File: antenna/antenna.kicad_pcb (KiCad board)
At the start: 2 copper layers, 50 x 43.3 mm, 24 parts, among them J1 Conn_01x05_Pin, J2 Conn_01x05_Pin, J3 Conn_01x05_Pin, J5 USB_C_Receptacle, SW1 SW_Push, SW2 SW_Push, U1 ESP32-C3-WROOM-02, U2 AMS1117-3.3

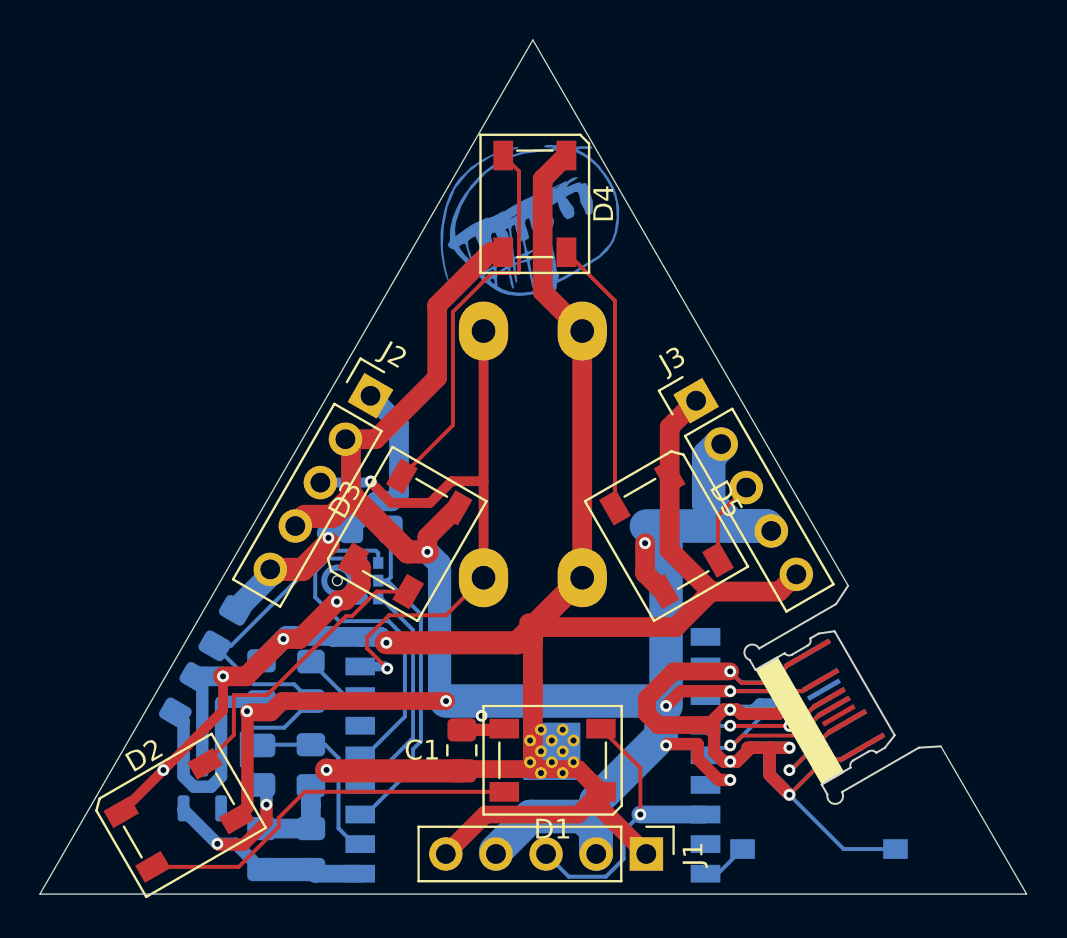
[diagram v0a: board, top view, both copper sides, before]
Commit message: url-update and some bla
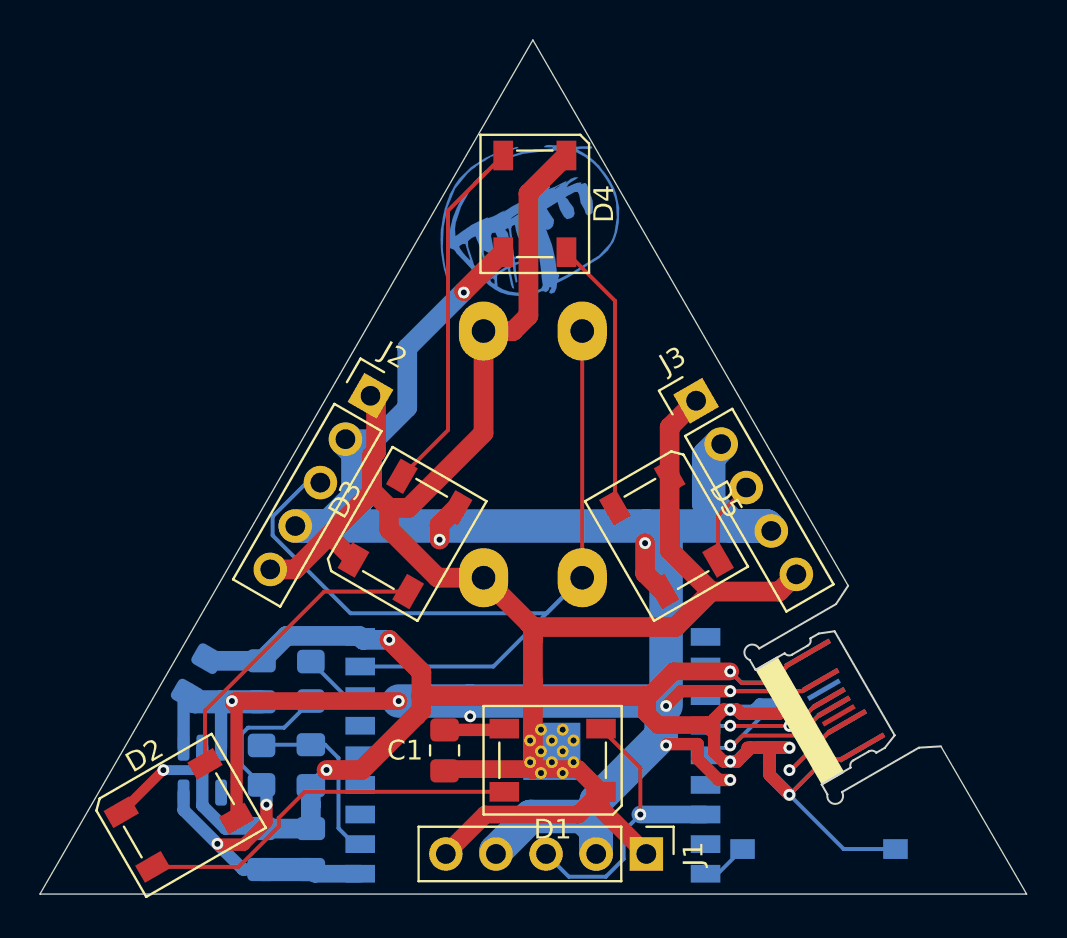
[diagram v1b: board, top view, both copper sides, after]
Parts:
- removed C7: 4u7F, Capacitor_SMD:C_0805_2012Metric_Pad1.18x1.45mm_HandSolder
- removed MK1: ICS-43434, Sensor_Audio:InvenSense_ICS-43434-6_3.5x2.65mm
- removed R3: 100k, Resistor_SMD:R_0805_2012Metric_Pad1.20x1.40mm_HandSolder
- moved SW1 13.5 mm to (147.5, 64.8), turned to -90 degrees
- moved C4 1.12 mm to (133.0, 82.2)
- moved C1 0.87 mm to (145.5, 86.0)
- moved U2 0.80 mm to (133.2, 87.0)
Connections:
- net +3.3V renamed Net-(U1-3V3)
- D1 pad 2: GND -> Net-(D1-DIN)
- J1 pad 3: GND -> Net-(D1-DIN)
- SW2 pad 1: Net-(U1-IO0) -> GND
- SW2 pad 2: GND -> Net-(U1-IO0)
- U1 pad 16: GND -> Net-(D1-DIN)
- U1 pad 3: Net-(MK1-SD) -> unconnected-(U1-IO4-Pad3)
- U1 pad 4: Net-(MK1-WS) -> unconnected-(U1-IO5-Pad4)
- U1 pad 5: Net-(MK1-SCK) -> unconnected-(U1-IO6-Pad5)
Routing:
- net Net-(MK1-SD): track 17.6 -> 0.00 mm
- net Net-(MK1-SCK): track 16.5 -> 0.00 mm
- net Net-(U1-3V3): track 39.4 -> 23.3 mm
- net Net-(D1-DIN): track 0.00 -> 15.9 mm, vias 0 -> 1
- net GND: track 218.2 -> 205.3 mm, vias 14 -> 9
- net Net-(MK1-WS): track 11.6 -> 0.00 mm
- net +5V: track 139.4 -> 142.7 mm, vias 10 -> 11
- net Net-(J2-Pin_3): track 44.8 -> 47.8 mm, vias 2 -> 0
- net Net-(D3-DOUT): track 19.8 -> 18.4 mm
